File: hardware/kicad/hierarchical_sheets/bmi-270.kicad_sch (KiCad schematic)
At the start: 4 parts

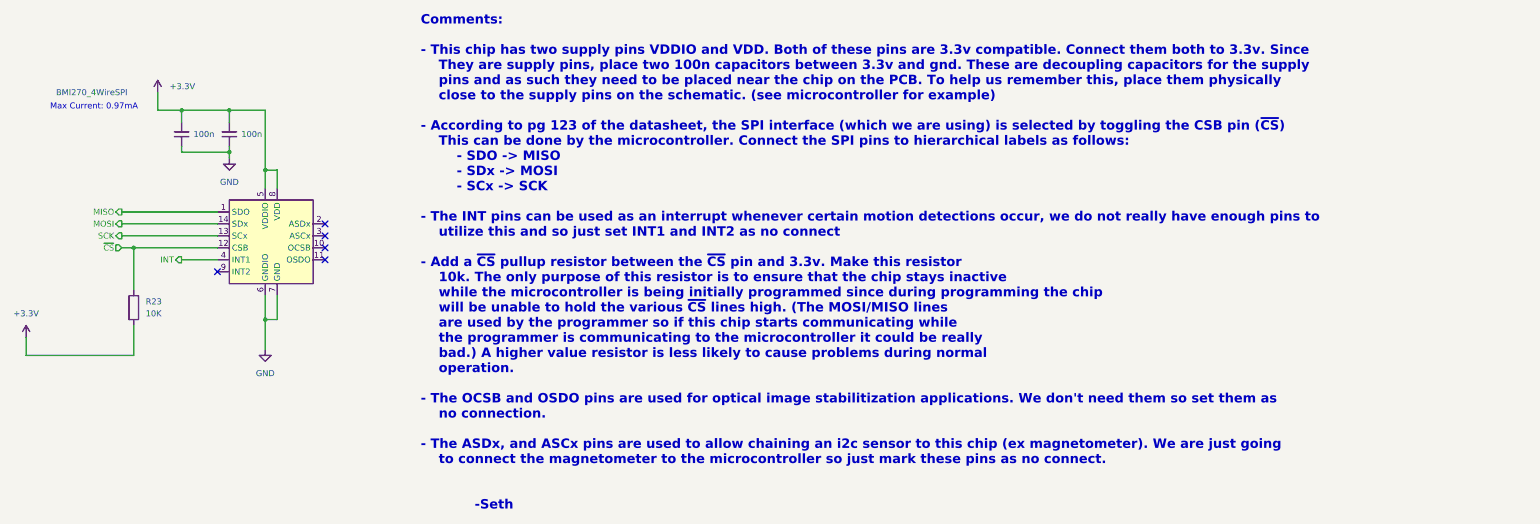
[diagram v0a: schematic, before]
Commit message: added power and checked schematics
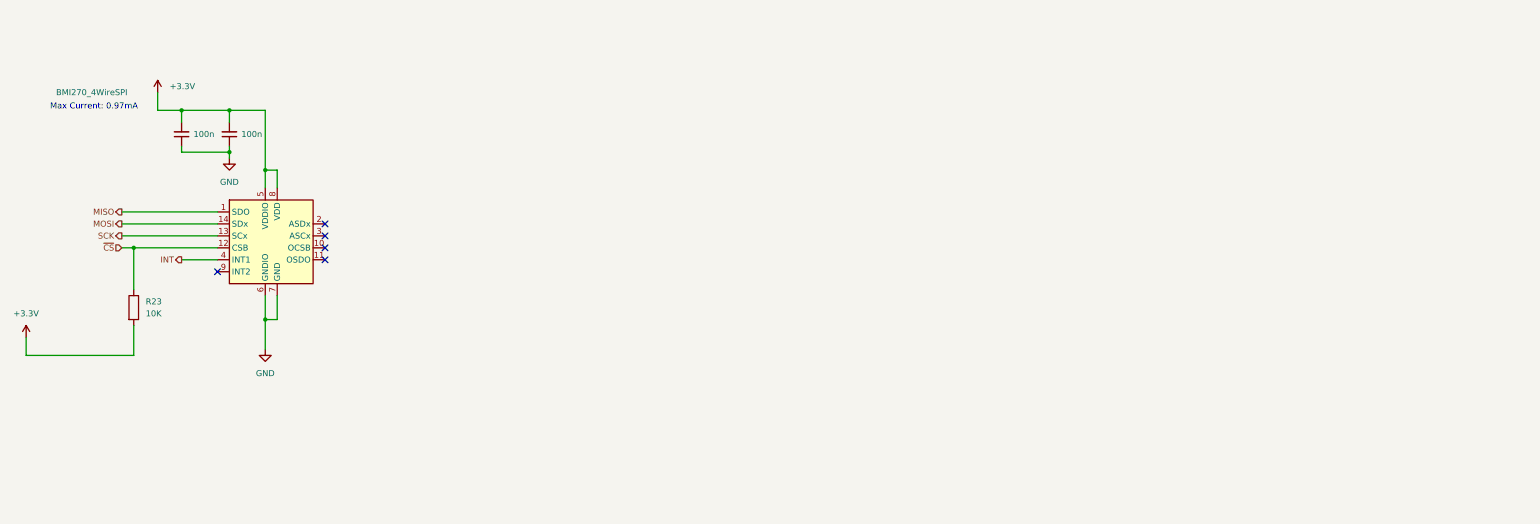
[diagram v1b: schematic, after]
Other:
- note removed: "Comments: - This chip has two supply pins VDDIO and VDD. Both of these pins are 3.3v compatible. Connect them both to 3.3v. Since They are supply pins, place two 100n capacitors between 3.3v and gnd. These are decoupling capacitors for the supply pins and as such they need to be placed near the chip on the PCB. To help us remember this, place them physically close to the supply pins on the schema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"
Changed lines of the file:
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@@
     (effects (font (size 1.27 1.27)) (justify left bottom))
-  )
-  (text "Comments:\n\n- This chip has two supply pins VDDIO and VDD. Both of these pins are 3.3v compatible. Connect them both to 3.3v. Since\n	They are supply pins, place two 100n capacitors between 3.3v and gnd. These are decoupling capacitors for the supply\n	pins and as such they need to be placed near the chip on the PCB. To help us remember this, place them physically\n	close to the supply pins on the schematic. (see microcontroller for example) \n\n- According to pg 123 of the datasheet, the SPI interface (which we are using) is selected by toggling the CSB pin (~{CS})\n	This can be done by the microcontroller. Connect the SPI pins to hierarchical labels as follows:\n		- SDO -> MISO\n		- SDx -> MOSI\n		- SCx -> SCK\n\n- The INT pins can be used as an interrupt whenever certain motion detections occur, we do not really have enough pins to \n	utilize this and so just set INT1 and INT2 as no connect\n\n- Add a ~{CS} pullup resistor between the ~{CS} pin and 3.3v. Make this resistor\n	10k. The only purpose of this resistor is to ensure that the chip stays inactive \n	while the microcontroller is being initially programmed since during programming the chip\n	will be unable to hold the various ~{CS} lines high. (The MOSI/MISO lines \n	are used by the programmer so if this chip starts communicating while\n	the programmer is communicating to the microcontroller it could be really \n	bad.) A higher value resistor is less likely to cause problems during normal \n	operation. \n\n- The OCSB and OSDO pins are used for optical image stabilitization applications. We don't need them so set them as\n	no connection.  \n\n- The ASDx, and ASCx pins are used to allow chaining an i2c sensor to this chip (ex magnetometer). We are just going\n	to connect the magnetometer to the microcontroller so just mark these pins as no connect. \n\n\n			-Seth"
-    (at 162.56 160.02 0)
-    (effects (font (size 2 2) (thickness 0.4) bold (color 255 48 0 1)) (justify left bottom))
   )
   (hierarchical_label "INT" (shape output) (at 111.76 106.68 180) (fields_autoplaced)
